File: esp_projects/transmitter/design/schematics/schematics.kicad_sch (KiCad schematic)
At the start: 6 parts, among them U1 CD4053B, U3 XIAO-ESP32-C3-DIP

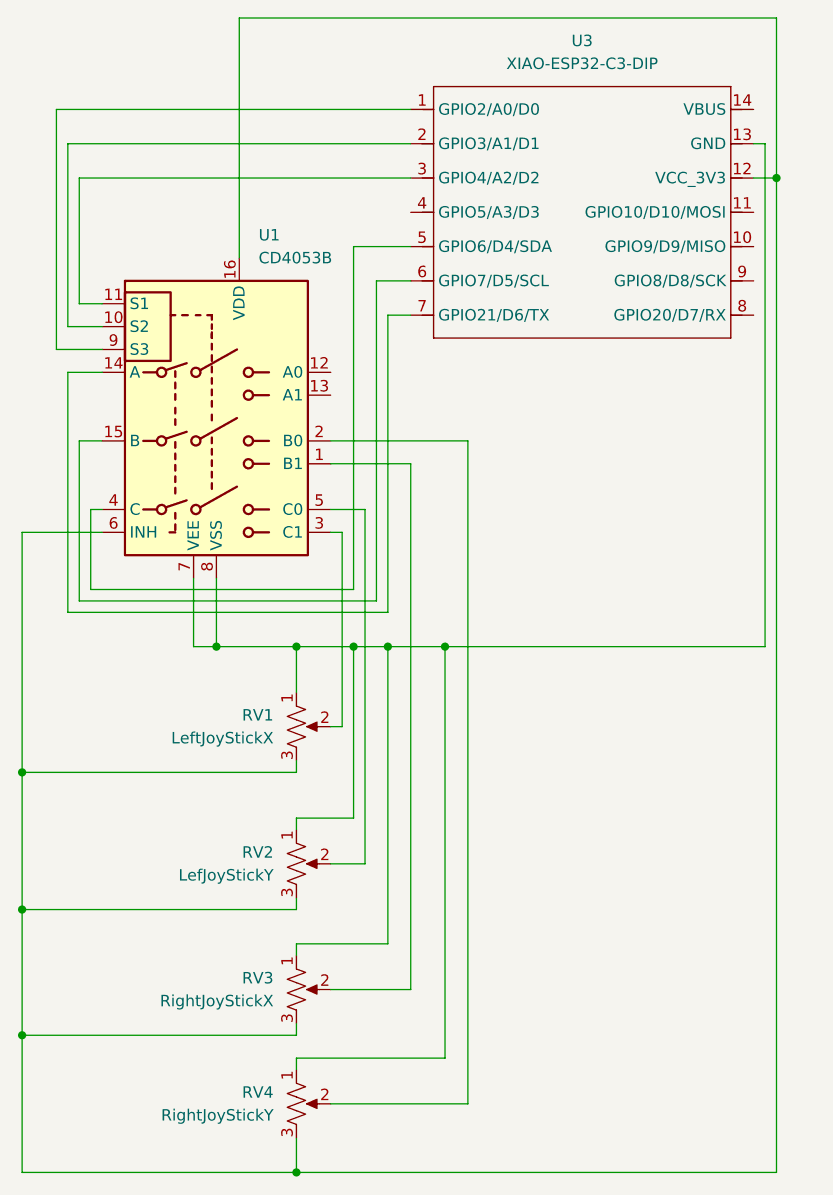
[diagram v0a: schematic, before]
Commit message: Add Schematics
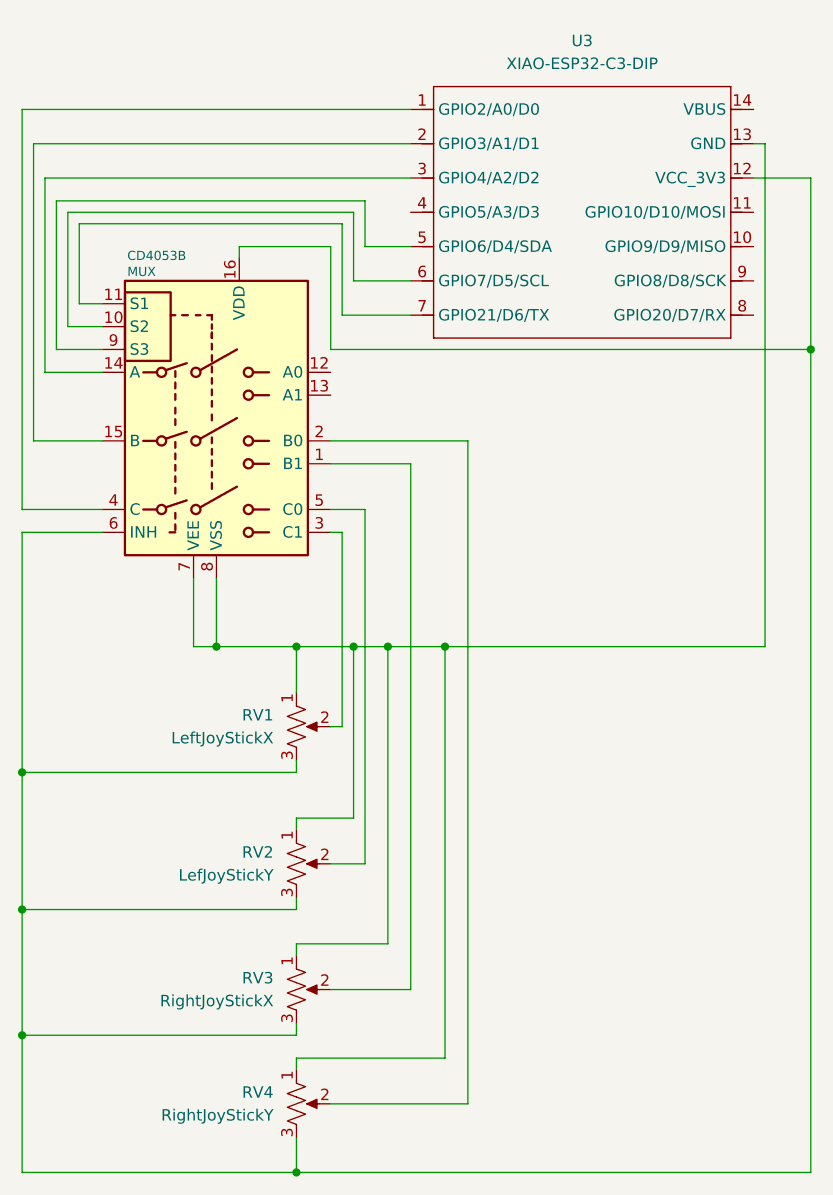
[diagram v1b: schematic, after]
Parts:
- renumbered U1 to MUX
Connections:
- net at MUX.10 (S2): now also U3.6 (GPIO7/D5/SCL); no longer U3.2 (GPIO3/A1/D1)
- net at MUX.11 (S1): now also U3.7 (GPIO21/D6/TX); no longer U3.3 (GPIO4/A2/D2)
- net at MUX.14 (A): now also U3.3 (GPIO4/A2/D2); no longer U3.7 (GPIO21/D6/TX)
- net at MUX.15 (B): now also U3.2 (GPIO3/A1/D1); no longer U3.6 (GPIO7/D5/SCL)
- net at MUX.4 (C): now also U3.1 (GPIO2/A0/D0); no longer U3.5 (GPIO6/D4/SDA)
- net at MUX.9 (S3): now also U3.5 (GPIO6/D4/SDA); no longer U3.1 (GPIO2/A0/D0)
